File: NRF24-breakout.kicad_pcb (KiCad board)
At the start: 2 copper layers, 27.3 x 22.9 mm, 2 parts, among them J1 CONN_01X08, U1 nRF24

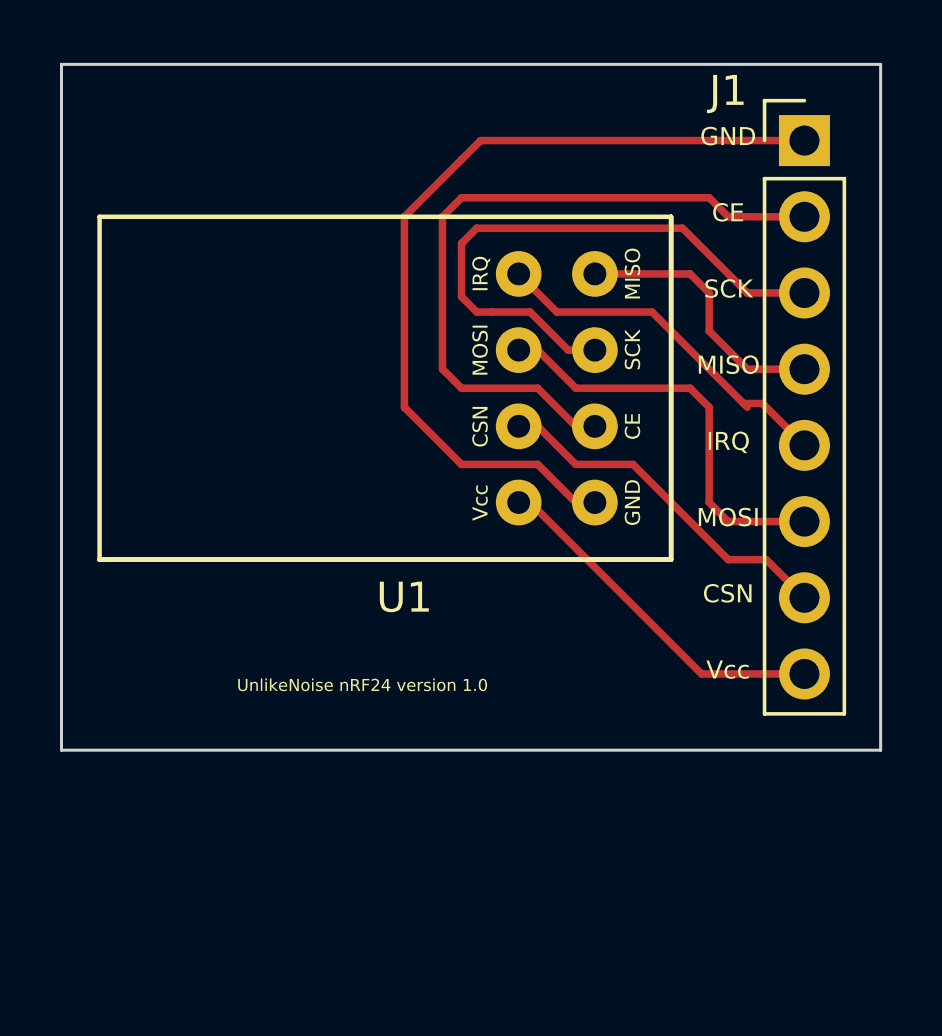
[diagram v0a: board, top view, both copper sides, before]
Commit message: Update Pcbnew with the new netlist
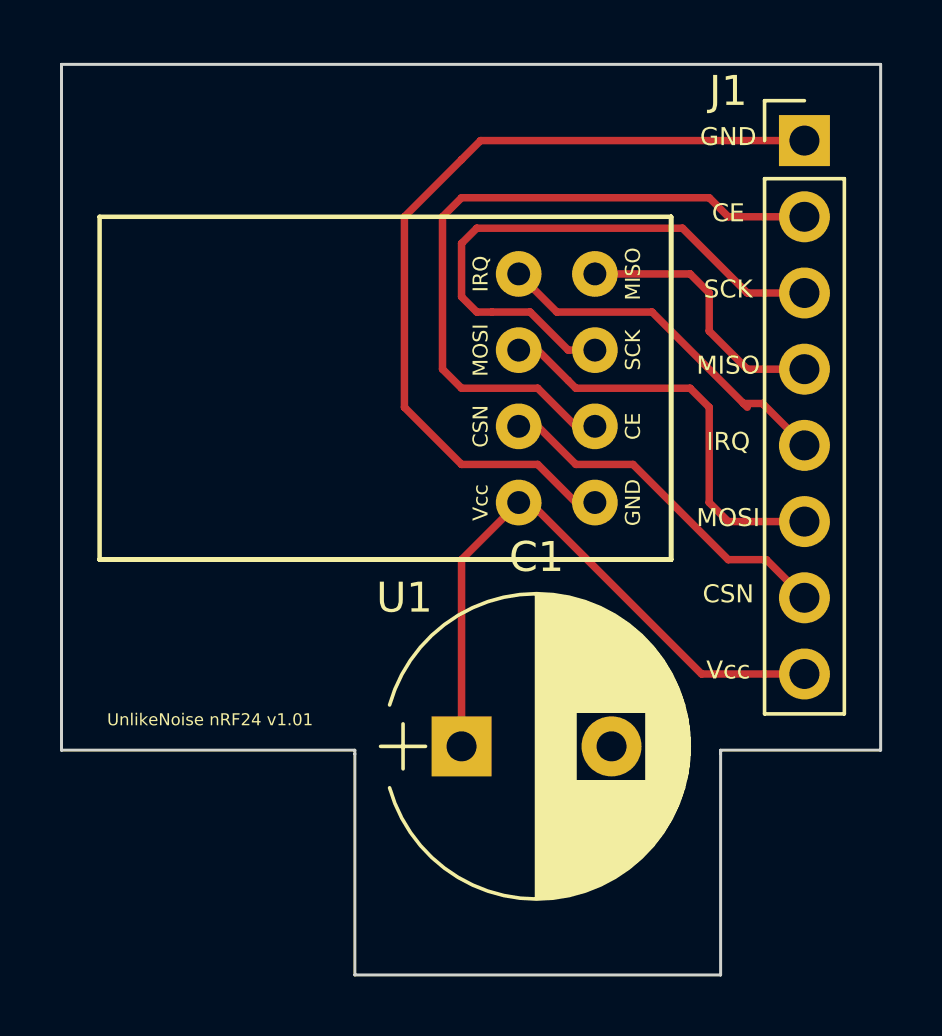
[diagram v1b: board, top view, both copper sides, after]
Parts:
- added C1: 10uF, Capacitors_THT:CP_Radial_D10.0mm_P5.00mm, F.Cu at (142.2, 137.7)
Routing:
- net Net-(C1-Pad1): track 11.9 -> 20.8 mm
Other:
- board size 27.3 x 22.9 mm -> 27.3 x 30.4 mm
- board text added: "UnlikeNoise nRF24 v1.01"
- board text removed: "UnlikeNoise nRF24 version 1.0"
